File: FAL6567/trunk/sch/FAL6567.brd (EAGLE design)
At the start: 97.5 x 77.5 mm, 20 parts, among them IC1 74LS245DW, IC2 74LS245DW, IC3 74LS245DW, IC4 74LS245DW, IC5 74LS06D

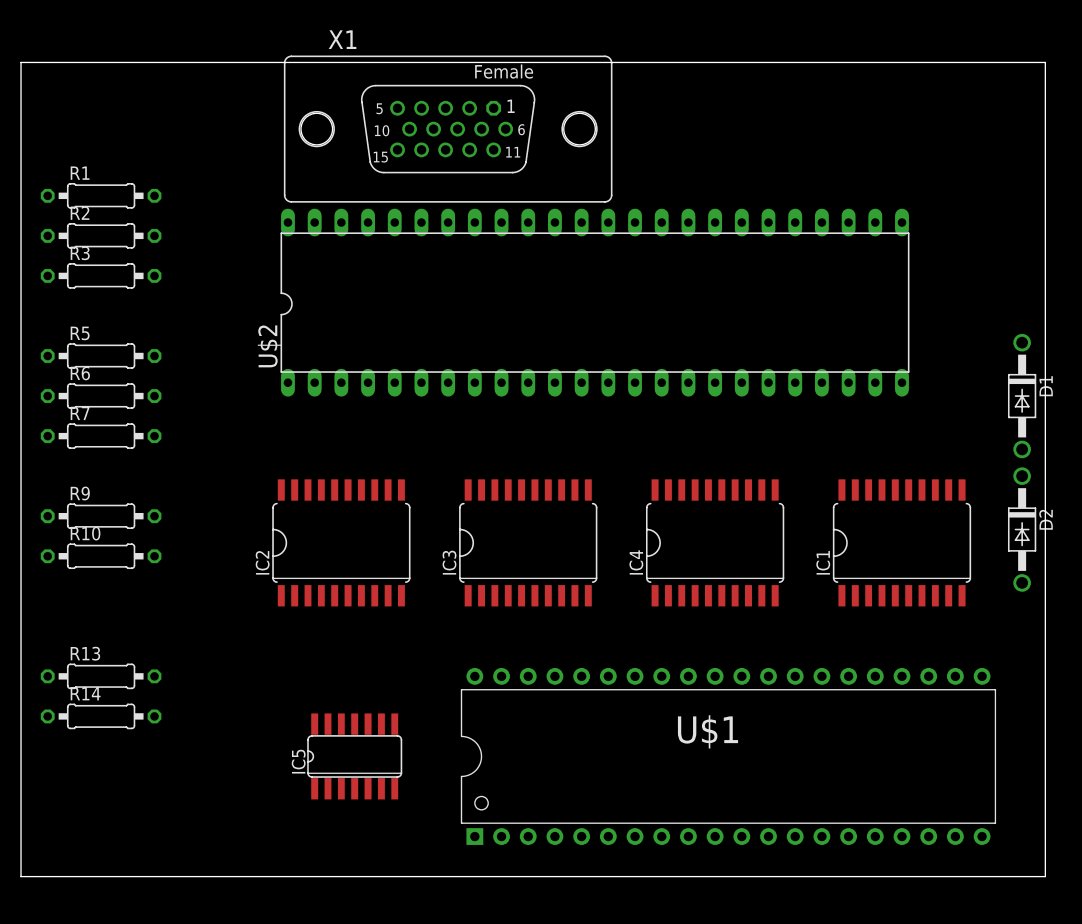
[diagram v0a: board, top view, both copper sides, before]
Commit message: FAL6567 - Latest Files
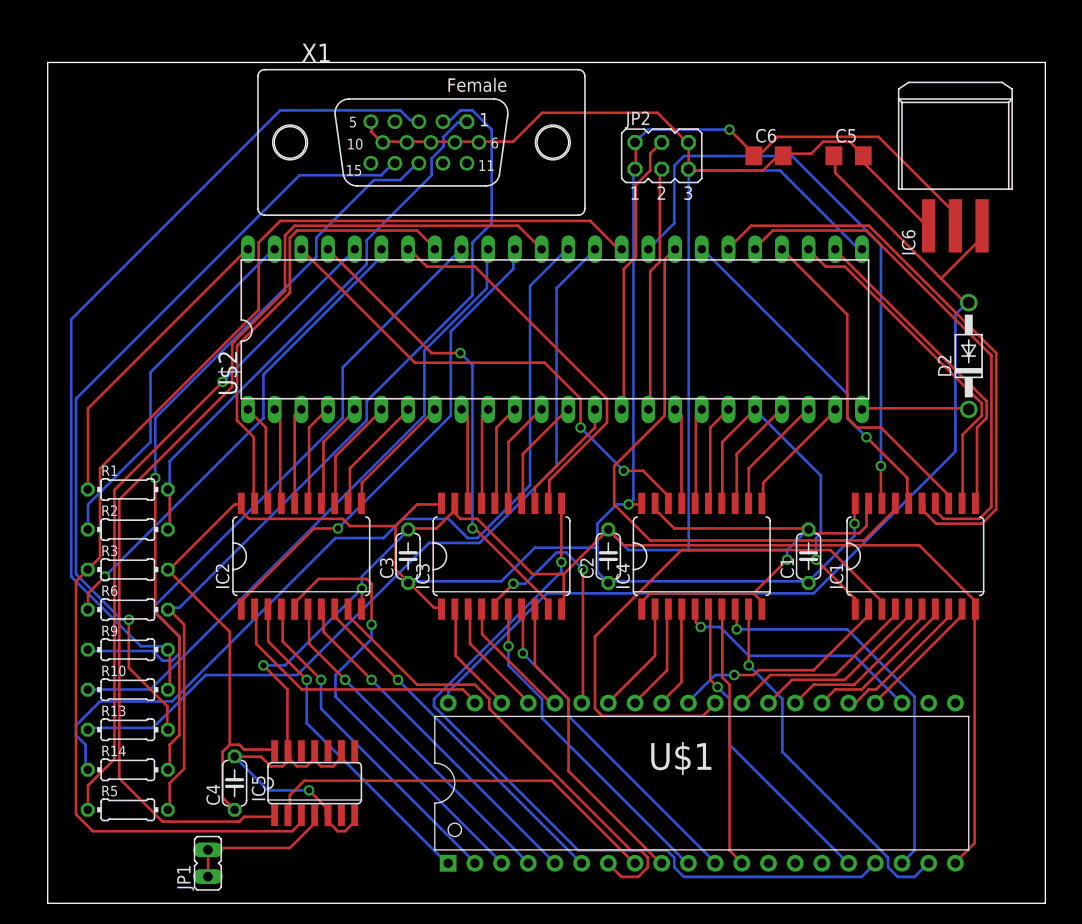
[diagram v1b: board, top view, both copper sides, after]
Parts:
- removed D1: 1N4004, diode:DO41-10
- removed R7: 510, resistor:0207/10
- added C1, C2, C3: (no value), resistor:C050-024X044
- added C4: 0.1, resistor:C050-024X044
- added C5, C6: 10u, resistor:C1206
- added IC6: REG1117F, burr-brown:DD-3
- added JP1: (no value), jumper:JP1
- added JP2: (no value), jumper:JP3Q
- R1, R5: value 2k -> 1k; device resistor:0207/10 -> resistor:0204/7
- R10, R13, R14, R9: device resistor:0207/10 -> resistor:0204/7
- R2, R6: value 1k -> 510; device resistor:0207/10 -> resistor:0204/7
- R3: value 510 -> 4.7k; device resistor:0207/10 -> resistor:0204/7
- moved R5 43.3 mm to (12.7, 8.89)
- moved R1 28.1 mm to (12.7, 39.4)
- moved R2 28.1 mm to (12.7, 35.6)
- moved R3 28.1 mm to (12.7, 31.8)
- moved R6 20.5 mm to (12.7, 27.9)
- moved D2 17.3 mm to (92.7, 52.1), turned to 90 degrees
- moved R10 13.0 mm to (12.7, 20.3)
- moved R9 13.0 mm to (12.7, 24.1)
- moved R14 5.68 mm to (12.7, 12.7)
- moved R13 5.68 mm to (12.7, 16.5)
- moved IC5 4.58 mm to (30.5, 11.4)
- moved U$2 4.58 mm to (53.3, 54.6)
- moved IC2 4.02 mm to (29.2, 33.0)
- moved U$1 3.59 mm to (66.0, 11.4)
- moved IC3 2.84 mm to (48.3, 33.0)
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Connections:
- removed net +3V3: IC3.1
- removed net GREEN2: R7.1, U$2.42
- removed net N$2: U$2.25
- removed net N$3: D1.C, U$2.24
- removed net N$6: D1.A, D2.C
- removed net RED2: R3.1, U$2.46
- new net MD0: JP2.4, U$2.15
- new net MD1: JP2.3, U$2.16
- new net N$8: IC5.4, JP1.1, JP1.2
- net +5V: now also C5.1, IC6.3
- net A10: now also U$2.46; no longer U$2.16
- net GND: now also C1.2, C2.2, C3.2, C4.2, C5.2, C6.2, IC5.11, IC5.13, IC5.5, IC5.9, IC6.1, JP2.5, JP2.6, U$2.25
- net LPB: now also U$2.42; no longer U$2.15
- net N$15: no longer R7.2
- net N$4: now also D2.C, U$2.24; no longer IC5.4
- net N$7: no longer R3.2
- net RESET: now also R3.1
- net VA1: now also U$1.25
- net VCC: now also C1.1, C2.1, C3.1, C4.1, C6.1, IC3.1, IC6.2, JP2.1, JP2.2, R3.2
- net VD3: now also IC2.6
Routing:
- net GND: track 0.00 -> 339.7 mm, vias 0 -> 4
- net VCC: track 0.00 -> 202.4 mm, vias 0 -> 3
- net RESET: track 0.00 -> 121.3 mm
- net IRQ: track 0.00 -> 100.6 mm
- net +5V: track 0.00 -> 99.7 mm
- net N$15: track 0.00 -> 85.3 mm
- net HSYNC: track 0.00 -> 82.9 mm
- net N$10: track 0.00 -> 82.4 mm
- net VSYNC: track 0.00 -> 77.2 mm
- net N$13: track 0.00 -> 75.1 mm, vias 0 -> 1
- net VPHI02: track 0.00 -> 74.1 mm, vias 0 -> 1
- net N$12: track 0.00 -> 71.1 mm, vias 0 -> 1
- net GREEN0: track 0.00 -> 63.9 mm, vias 0 -> 1
- net BLUE1: track 0.00 -> 61.2 mm
- net BLUE0: track 0.00 -> 61.0 mm
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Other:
- board size 97.5 x 77.5 mm -> 94.9 x 80 mm
